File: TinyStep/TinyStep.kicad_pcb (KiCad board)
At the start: 2 copper layers, 17.8 x 25.4 mm, 2 parts, among them U1 ATtiny204-SS

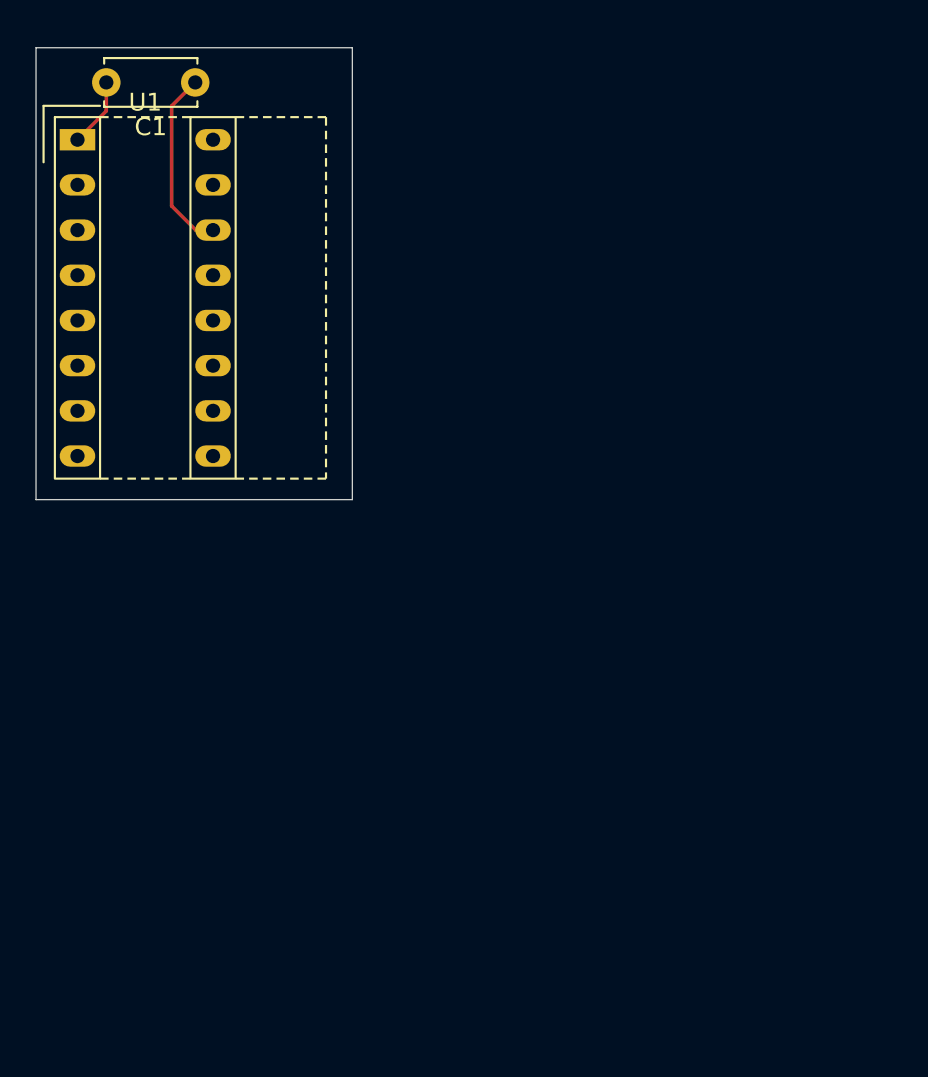
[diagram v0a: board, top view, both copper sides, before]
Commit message: this might work
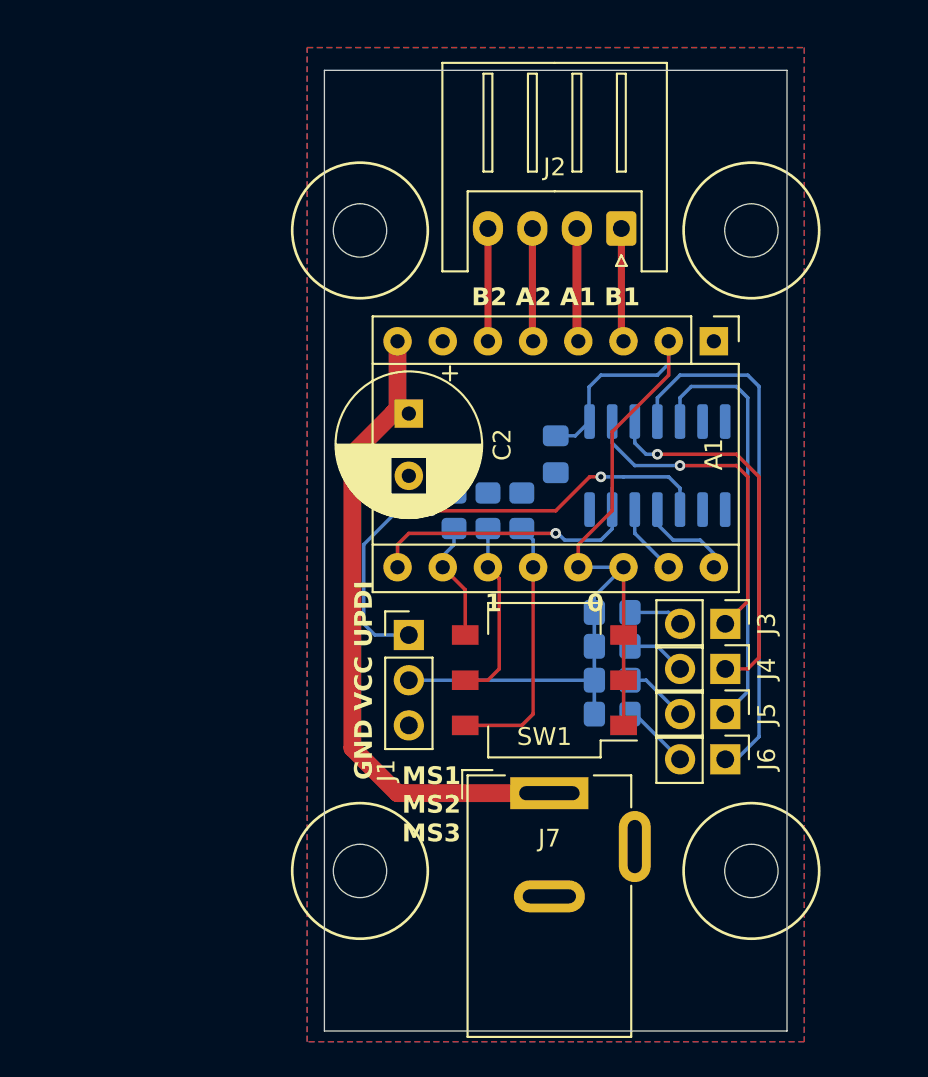
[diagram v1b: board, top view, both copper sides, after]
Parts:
- added A1: Pololu_Breakout_A4988, Module:Pololu_Breakout-16_15.2x20.3mm, F.Cu at (57.1, 35.5)
- added C2: 100uF 50V, Capacitor_THT:CP_Radial_D8.0mm_P3.50mm, F.Cu at (40.0, 39.6)
- added J1: Conn_01x03_Pin, Connector_PinHeader_2.54mm:PinHeader_1x03_P2.54mm_Vertical, F.Cu at (40.0, 52.1)
- added J2: Conn_01x04_Pin, Connector_JST:JST_XH_S4B-XH-A_1x04_P2.50mm_Horizontal, F.Cu at (52.0, 29.2)
- added J3: Conn_01x02_Pin, Connector_PinHeader_2.54mm:PinHeader_1x02_P2.54mm_Vertical, F.Cu at (57.8, 51.4)
- added J4: Conn_01x02_Pin, Connector_PinHeader_2.54mm:PinHeader_1x02_P2.54mm_Vertical, F.Cu at (57.8, 54.0)
- added J5: Conn_01x02_Pin, Connector_PinHeader_2.54mm:PinHeader_1x02_P2.54mm_Vertical, F.Cu at (57.8, 56.5)
- added J6: Conn_01x02_Pin, Connector_PinHeader_2.54mm:PinHeader_1x02_P2.54mm_Vertical, F.Cu at (57.8, 59.0)
- added J7: Barrel_Jack_Switch, Connector_BarrelJack:BarrelJack_Wuerth_6941xx301002, F.Cu at (47.9, 61.0)
- added R1: 10k, Resistor_SMD:R_0805_2012Metric_Pad1.20x1.40mm_HandSolder, B.Cu at (46.4, 45.1)
- added R2: 10k, Resistor_SMD:R_0805_2012Metric_Pad1.20x1.40mm_HandSolder, B.Cu at (44.5, 45.1)
- added R3: 10k, Resistor_SMD:R_0805_2012Metric_Pad1.20x1.40mm_HandSolder, B.Cu at (42.5, 45.1)
- added R4: 10k, Resistor_SMD:R_0805_2012Metric_Pad1.20x1.40mm_HandSolder, B.Cu at (51.4, 50.8)
- added R5: 10k, Resistor_SMD:R_0805_2012Metric_Pad1.20x1.40mm_HandSolder, B.Cu at (51.4, 52.7)
- added R6: 10k, Resistor_SMD:R_0805_2012Metric_Pad1.20x1.40mm_HandSolder, B.Cu at (51.4, 54.6)
- added R7: 10k, Resistor_SMD:R_0805_2012Metric_Pad1.20x1.40mm_HandSolder, B.Cu at (51.4, 56.5)
- added SW1: SW_DIP_x03, Button_Switch_SMD:SW_DIP_SPSTx03_Slide_Omron_A6S-310x_W8.9mm_P2.54mm, F.Cu at (47.6, 54.6)
- C1: value C -> 100n; footprint Capacitor_THT:C_Disc_D5.0mm_W2.5mm_P5.00mm -> Capacitor_SMD:C_0805_2012Metric_Pad1.18x1.45mm_HandSolder; moved to B.Cu
- U1: footprint BREAKOUT:DIP-16_SOIC_BREAKOUT -> Package_SO:SOIC-14_3.9x8.7mm_P1.27mm; moved to B.Cu
- moved U1 37.4 mm to (54.0, 42.5), turned to -90 degrees
- moved C1 29.1 mm to (48.3, 41.9), turned to 90 degrees
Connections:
- net Net-(U1-GND) renamed GND
- U1 pad 10: unconnected-(U1-~{RESET}/PA0-Pad10) -> UPDI
- U1 pad 11: unconnected-(U1-PA1-Pad11) -> A1_DI
- U1 pad 12: unconnected-(U1-PA2-Pad12) -> A1_ST
- U1 pad 13: unconnected-(U1-PA3-Pad13) -> A1_EN
- U1 pad 2: unconnected-(U1-PA4-Pad2) -> BTN0
- U1 pad 3: unconnected-(U1-PA5-Pad3) -> BTN1
- U1 pad 4: unconnected-(U1-PA6-Pad4) -> BTN3
- U1 pad 5: unconnected-(U1-PA7-Pad5) -> BTN2
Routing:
- net VCC: track 3.89 -> 55.4 mm
- net +12V: track 0.00 -> 36.9 mm
- net BTN3: track 0.00 -> 30.0 mm
- net UPDI: track 0.00 -> 28.1 mm, vias 0 -> 2
- net BTN2: track 0.00 -> 23.3 mm
- net BTN1: track 0.00 -> 21.3 mm, vias 0 -> 1
- net BTN0: track 0.00 -> 18.4 mm, vias 0 -> 1
- net A1_EN: track 0.00 -> 16.3 mm, vias 0 -> 1
- net Net-(A1-MS3): track 0.00 -> 14.8 mm
- net GND: track 10.4 -> 0.00 mm
- net Net-(A1-MS2): track 0.00 -> 10.3 mm
- net Net-(A1-MS1): track 0.00 -> 6.77 mm
- net Net-(A1-1B): track 0.00 -> 6.40 mm
- net Net-(A1-1A): track 0.00 -> 6.38 mm
- net Net-(A1-2A): track 0.00 -> 6.37 mm
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- added copper zone on B.Cu, net GND
- added copper zone on F.Cu, net GND
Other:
- board size 17.8 x 25.4 mm -> 26 x 54 mm
- board text added: "1 0"
- board text added: "B2 A2 A1 B1"
- board text added: "GND VCC UPDI"
- board text added: "MS1 MS2 MS3"

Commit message: v0.1
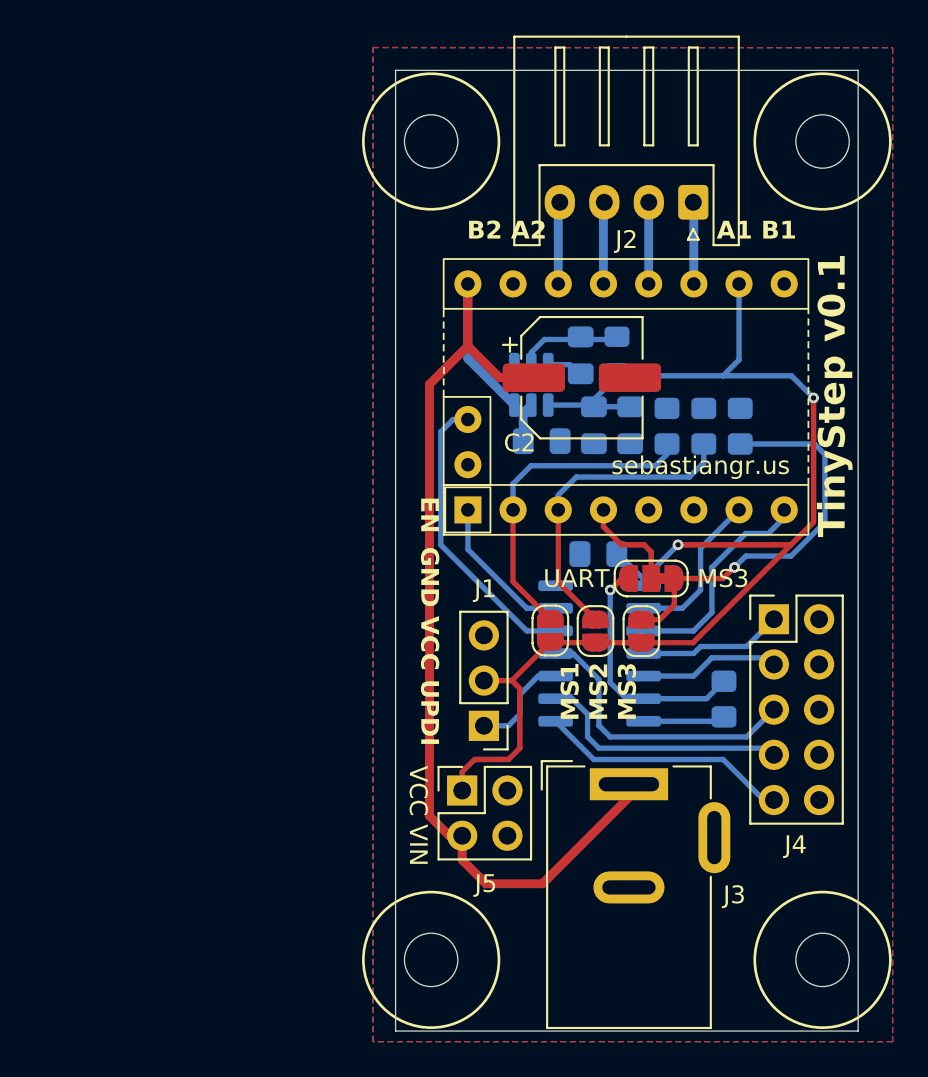
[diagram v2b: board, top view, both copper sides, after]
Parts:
- removed A1: Pololu_Breakout_A4988, Module:Pololu_Breakout-16_15.2x20.3mm
- removed the J3 at (57.8, 51.4)
- removed J6: Conn_01x02_Pin, Connector_PinHeader_2.54mm:PinHeader_1x02_P2.54mm_Vertical
- removed R5, R6, R7: 10k, Resistor_SMD:R_0805_2012Metric_Pad1.20x1.40mm_HandSolder
- removed SW1: SW_DIP_x03, Button_Switch_SMD:SW_DIP_SPSTx03_Slide_Omron_A6S-310x_W8.9mm_P2.54mm
- added A2: ~, Module_TMC2209_BTT:TMC2209_BTT, F.Cu at (52.2, 38.7)
- added C3: 10uF, Capacitor_SMD:C_0805_2012Metric_Pad1.18x1.45mm_HandSolder, B.Cu at (47.5, 41.2)
- added C4: 100nF, Capacitor_SMD:C_0805_2012Metric_Pad1.18x1.45mm_HandSolder, B.Cu at (49.7, 36.3)
- added C5: 22uF, Capacitor_SMD:C_0805_2012Metric_Pad1.18x1.45mm_HandSolder, B.Cu at (52.4, 40.3)
- added C6: 22uF, Capacitor_SMD:C_0805_2012Metric_Pad1.18x1.45mm_HandSolder, B.Cu at (50.4, 40.3)
- added JP1: SolderJumper_3_Bridged12, Jumper:SolderJumper-3_P1.3mm_Bridged12_RoundedPad1.0x1.5mm_NumberLabels, F.Cu at (53.6, 48.9)
- added JP2: SolderJumper_2_Open, Jumper:SolderJumper-2_P1.3mm_Open_RoundedPad1.0x1.5mm, F.Cu at (53.1, 51.8)
- added JP3: SolderJumper_2_Open, Jumper:SolderJumper-2_P1.3mm_Open_RoundedPad1.0x1.5mm, F.Cu at (50.5, 51.8)
- added JP4: SolderJumper_2_Open, Jumper:SolderJumper-2_P1.3mm_Open_RoundedPad1.0x1.5mm, F.Cu at (48.0, 51.8)
- added L1: 4.7uH, Inductor_SMD:L_0805_2012Metric_Pad1.15x1.40mm_HandSolder, B.Cu at (51.7, 36.3)
- added U2: AP63205WU, Package_TO_SOT_SMD:TSOT-23-6, B.Cu at (46.9, 38.0)
- C1: value 100n -> 100nF
- C2: value 100uF 50V -> 47uF 50V; footprint Capacitor_THT:CP_Radial_D8.0mm_P3.50mm -> Capacitor_SMD:CP_Elec_6.3x7.7
- J4: value Conn_01x02_Pin -> Conn_02x05_Odd_Even; footprint Connector_PinHeader_2.54mm:PinHeader_1x02_P2.54mm_Vertical -> Connector_PinHeader_2.54mm:PinHeader_2x05_P2.54mm_Vertical
- J5: value Conn_01x02_Pin -> Conn_02x02_Odd_Even; footprint Connector_PinHeader_2.54mm:PinHeader_1x02_P2.54mm_Vertical -> Connector_PinHeader_2.54mm:PinHeader_2x02_P2.54mm_Vertical
- R4: value 10k -> 1k
- moved R3 16.8 mm to (58.6, 40.3)
- moved J5 15.4 mm to (43.0, 60.8), turned to 0 degrees
- moved R2 13.0 mm to (56.6, 40.3)
- moved U1 11.1 mm to (50.7, 53.1), turned to 180 degrees
- moved C2 9.94 mm to (49.7, 37.6), turned to 0 degrees
- moved R1 9.44 mm to (54.5, 40.3)
- moved R4 7.95 mm to (57.7, 55.7), turned to 90 degrees
- moved J1 6.62 mm to (44.2, 57.2), turned to 180 degrees
- moved C1 6.10 mm to (50.7, 47.5), turned to 180 degrees
- moved J3 4.50 mm to (52.4, 60.4)
- moved J2 4.30 mm to (56.0, 27.7)
- moved J4 3.91 mm to (60.5, 51.2), turned to 0 degrees
- renumbered J7 to J3
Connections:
- C1 pad 1: GND -> VCC
- C1 pad 2: VCC -> GND
- J4 pad 1: BTN1 -> BTN0
- J4 pad 2: Net-(J4-Pin_2) -> GND
- J5 pad 1: BTN2 -> VCC
- J5 pad 2: Net-(J5-Pin_2) -> GND
- R3 pad 2: Net-(A1-MS1) -> A1_MS3_SW
- R4 pad 1: Net-(J3-Pin_2) -> /USART_Tx
- R4 pad 2: VCC -> A1_MS3_UART
- U1 pad 11: A1_DI -> BTN2
- U1 pad 12: A1_ST -> A1_DIAG
- U1 pad 2: BTN0 -> A1_ST
- U1 pad 3: BTN1 -> A1_DI
- U1 pad 4: BTN3 -> BTN0
- U1 pad 5: BTN2 -> BTN1
- U1 pad 6: unconnected-(U1-PB3-Pad6) -> A1_MS3_UART
- U1 pad 7: unconnected-(U1-PB2-Pad7) -> /USART_Tx
- U1 pad 8: unconnected-(U1-PB1-Pad8) -> BTN4
- U1 pad 9: unconnected-(U1-PB0-Pad9) -> BTN3
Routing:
- net +12V: track 36.9 -> 62.4 mm
- net UPDI: track 28.1 -> 5.84 mm, vias 2 -> 0
- net A1_MS3_SW: track 0.00 -> 22.3 mm, vias 0 -> 1
- net VCC: track 55.4 -> 73.3 mm, vias 0 -> 2
- net A1_DIAG: track 0.00 -> 16.6 mm
- net BTN3: track 30.0 -> 14.3 mm
- net BTN4: track 0.00 -> 14.1 mm
- net A1_MS3_UART: track 0.00 -> 13.6 mm, vias 0 -> 1
- net BTN1: track 21.3 -> 8.48 mm, vias 1 -> 0
- net BTN0: track 18.4 -> 8.65 mm, vias 1 -> 0
- net A1_EN: track 16.3 -> 8.52 mm, vias 1 -> 0
- net Net-(A2-MS2): track 10.3 -> 17.8 mm
- net BTN2: track 23.3 -> 16.4 mm
- net Net-(A1-MS1): track 6.77 -> 0.00 mm
- net A1_DI: track 6.15 -> 12.5 mm
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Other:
- outline, holes or cut-outs redrawn
- board text added: "MS3"
- board text added: "TinyStep v0.1"
- board text added: "UART"
- board text added: "VCC VIN"
- board text added: "sebastiangr.us"
- board text removed: "1 0"
